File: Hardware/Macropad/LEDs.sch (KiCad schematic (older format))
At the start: 62 parts

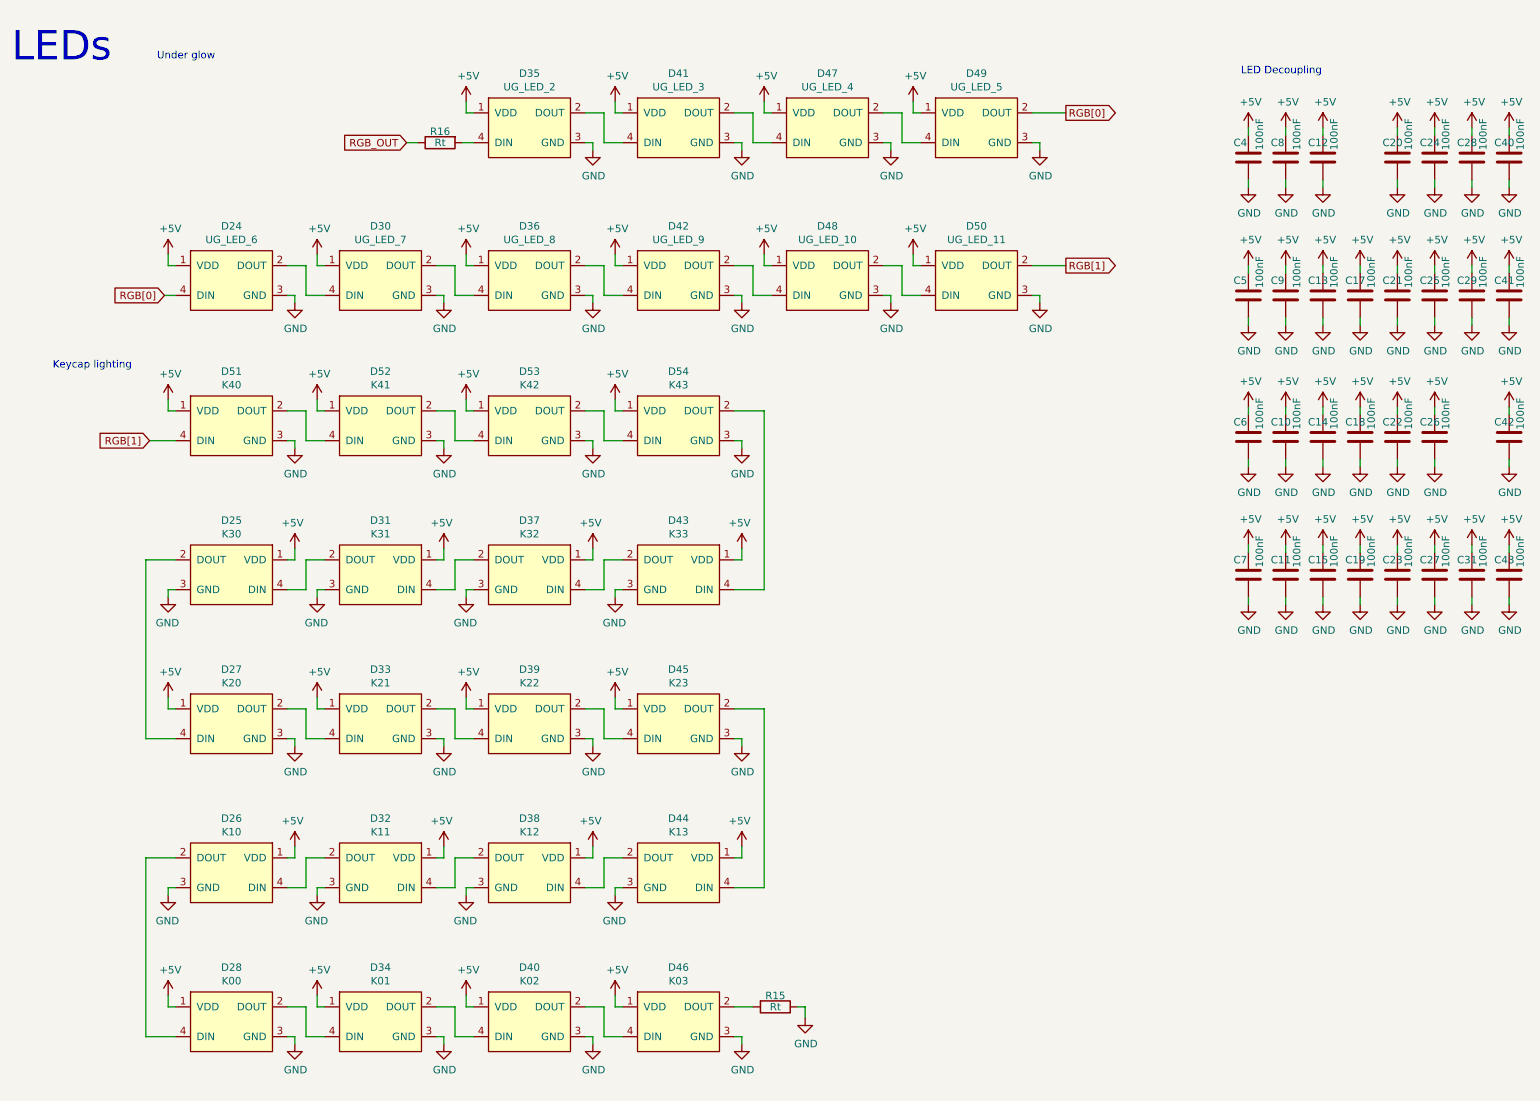
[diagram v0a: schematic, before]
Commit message: Layout done, cleaned up schematic and generated gerbers
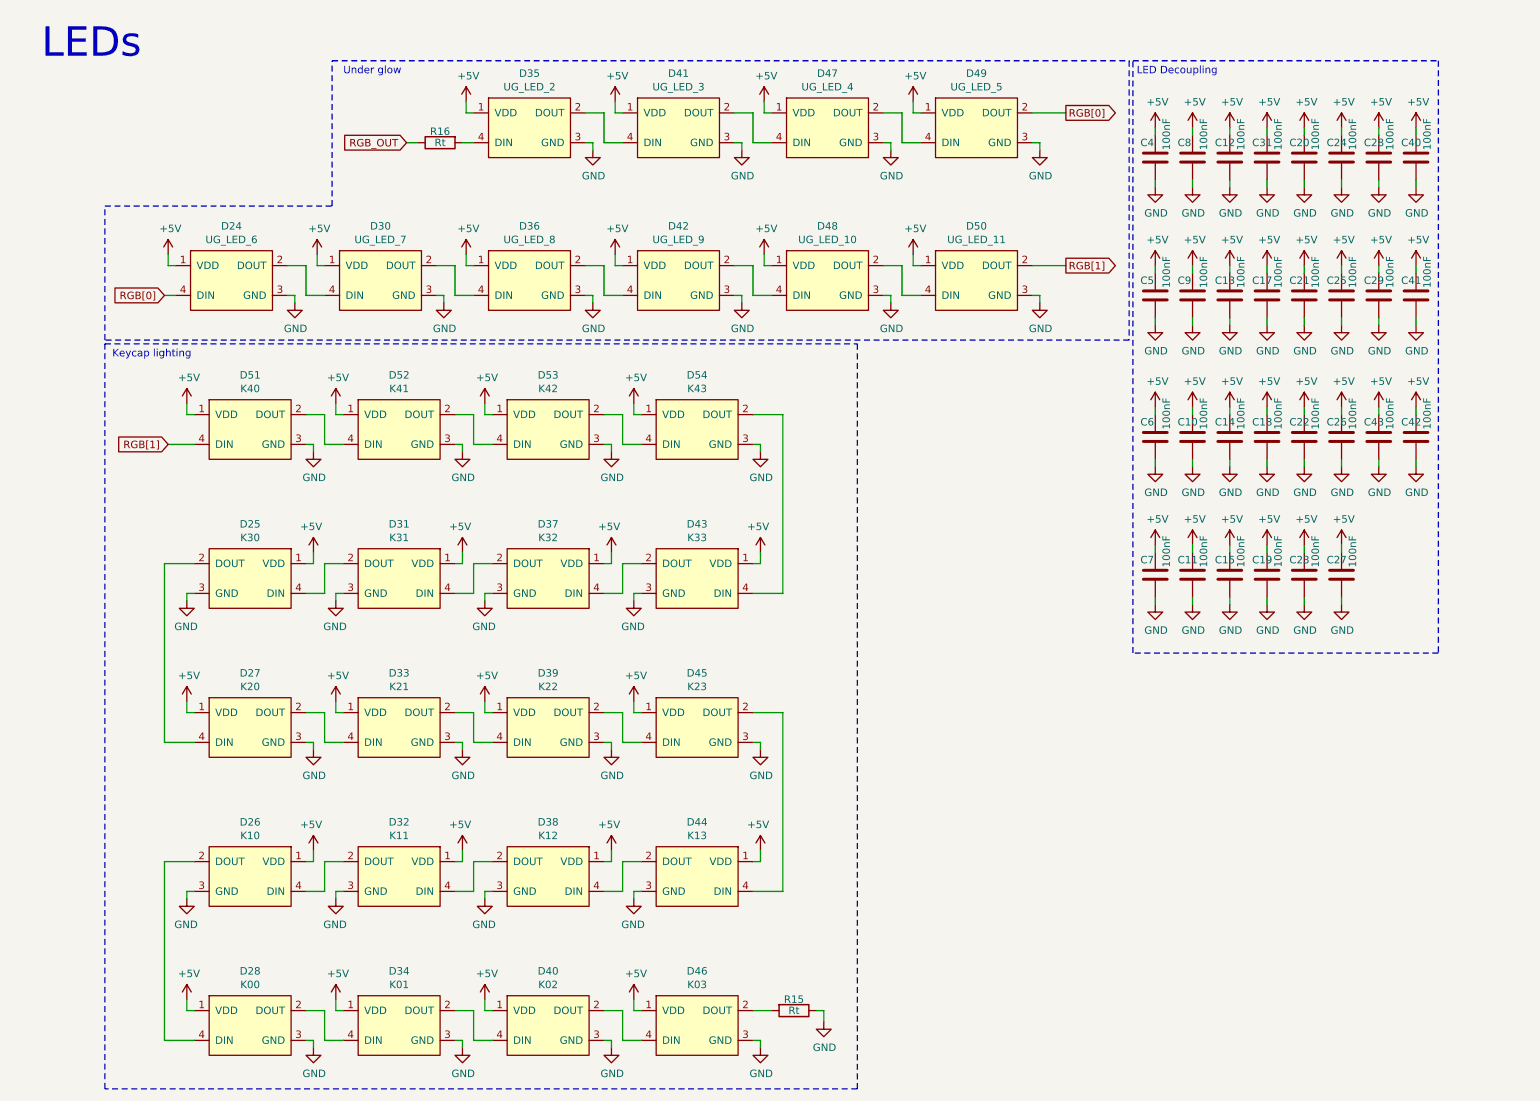
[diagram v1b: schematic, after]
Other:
- moved on the sheet: C10, C11, C12, C13, C14, C15, C17, C18, C19, C20, C21, C22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
